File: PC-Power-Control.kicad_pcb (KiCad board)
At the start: 2 copper layers, 48.5 x 23.7 mm, 10 parts, among them J1 Conn_02x06_Odd_Even

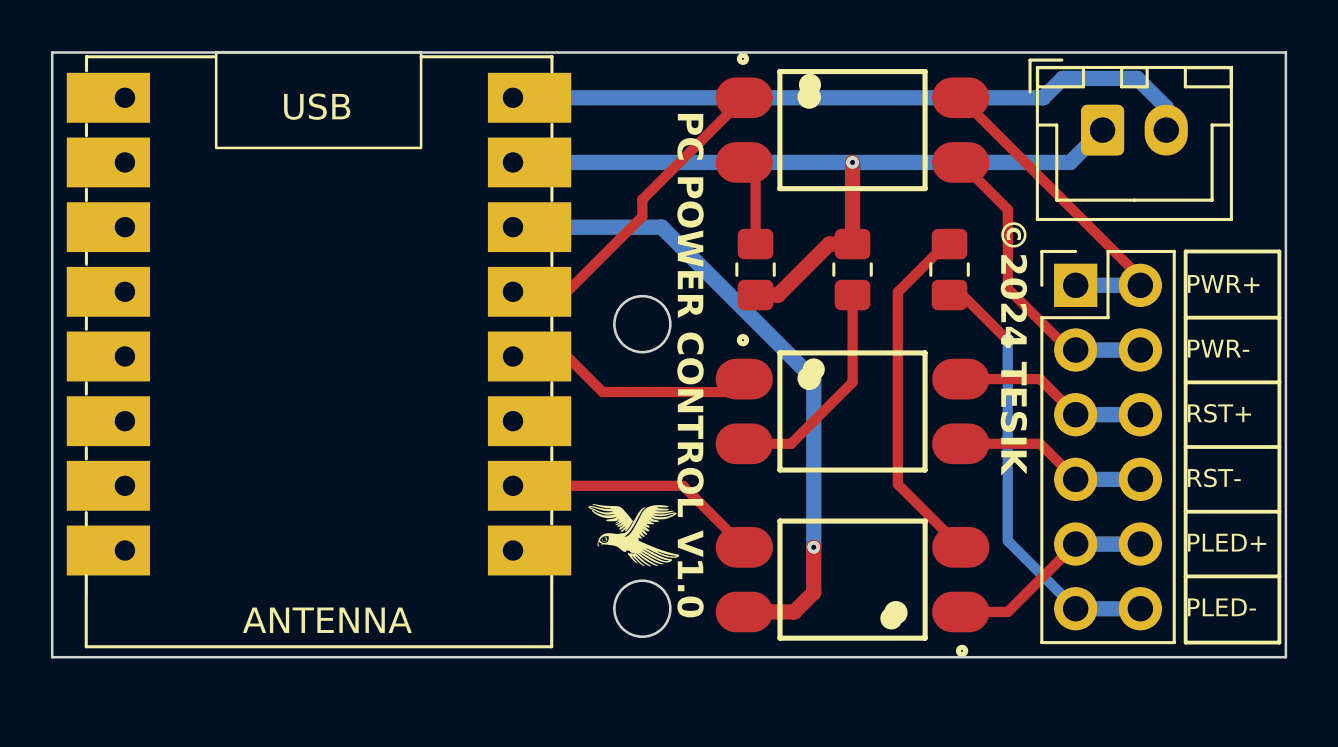
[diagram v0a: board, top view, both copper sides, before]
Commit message: update
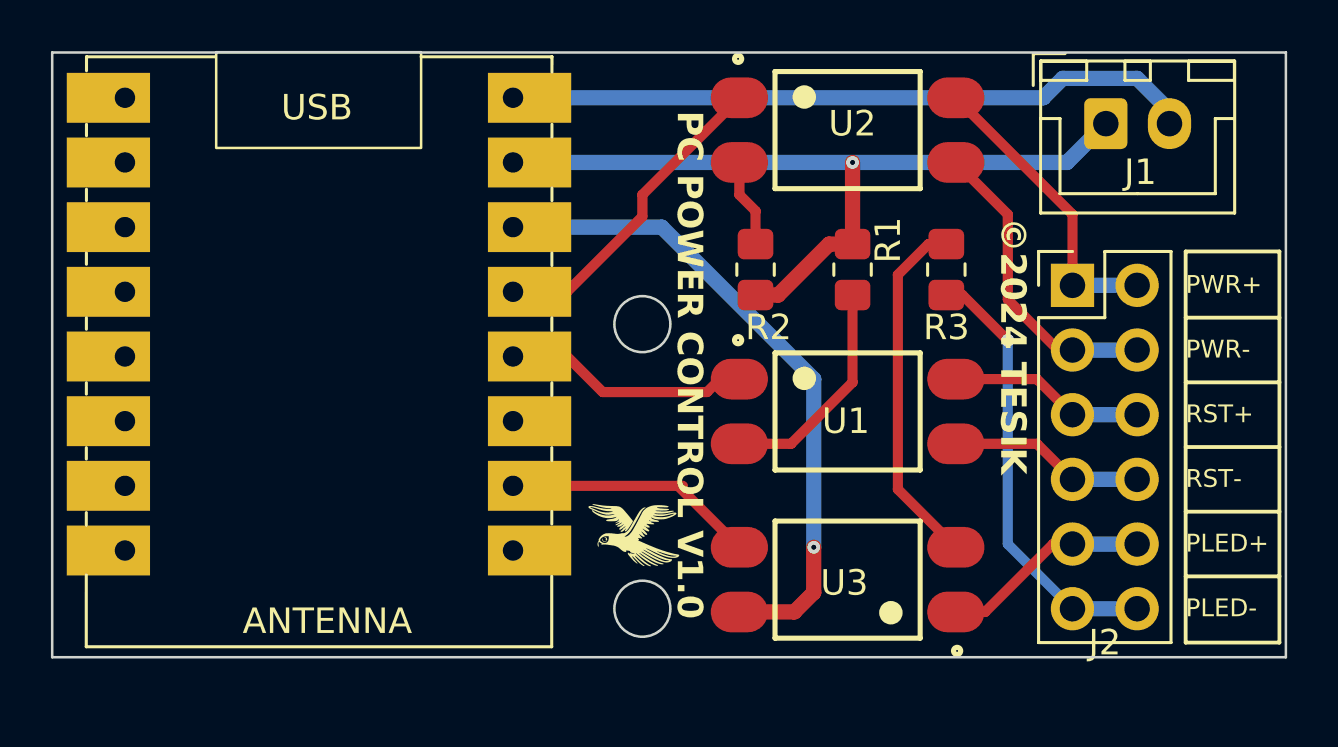
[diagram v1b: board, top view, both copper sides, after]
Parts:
- removed LED-RESISTOR1: R2K2, Resistor_SMD:R_0805_2012Metric_Pad1.20x1.40mm_HandSolder
- removed LED-SWITCH1, POWER-SWITCH1, RESET-SWITCH1: EL817, _jendova:SOT254P975X400-4N
- removed POWER-RESISTOR1, RESET-RESISTOR1: R330, Resistor_SMD:R_0805_2012Metric_Pad1.20x1.40mm_HandSolder
- removed POWER1: Conn_01x02, Connector_JST:JST_XH_B2B-XH-A_1x02_P2.50mm_Vertical
- added J2: Conn_02x06_Odd_Even, Connector_PinHeader_2.54mm:PinHeader_2x06_P2.54mm_Vertical, F.Cu at (85.7, 56.9)
- added R1: R330, Resistor_SMD:R_0805_2012Metric_Pad1.20x1.40mm_HandSolder, F.Cu at (77.1, 56.3)
- added R2: R330, Resistor_SMD:R_0805_2012Metric_Pad1.20x1.40mm_HandSolder, F.Cu at (73.3, 56.3)
- added R3: R2K2, Resistor_SMD:R_0805_2012Metric_Pad1.20x1.40mm_HandSolder, F.Cu at (80.8, 56.3)
- added U1: EL817, _jendova:SOT254P975X400-4N, F.Cu at (76.9, 61.8)
- added U2: EL817, _jendova:SOT254P975X400-4N, F.Cu at (76.9, 50.8)
- added U3: EL817, _jendova:SOT254P975X400-4N, F.Cu at (76.9, 68.5)
- J1: value Conn_02x06_Odd_Even -> Conn_01x02; footprint Connector_PinHeader_2.54mm:PinHeader_2x06_P2.54mm_Vertical -> Connector_JST:JST_XH_B2B-XH-A_1x02_P2.50mm_Vertical
- moved J1 6.46 mm to (87.0, 50.5)
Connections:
- J1 pad 1: Power + -> GND
- J1 pad 2: Power + -> +5V
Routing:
- net Power +: track 13.6 -> 11.8 mm
- net +5V: track 27.3 -> 28.0 mm
- net Reset Cathode: track 8.24 -> 8.87 mm
- net GPIO3: track 9.87 -> 10.4 mm
